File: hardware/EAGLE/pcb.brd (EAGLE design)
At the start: 17.8 x 110.5 mm, 44 parts, among them IC1 4017N, IC2 DG412DJD, IC3 DG412DJD, Q1 MMBT3904, Q2 MMBT3904, Q3 MMBT3904, Q4 MMBT3904

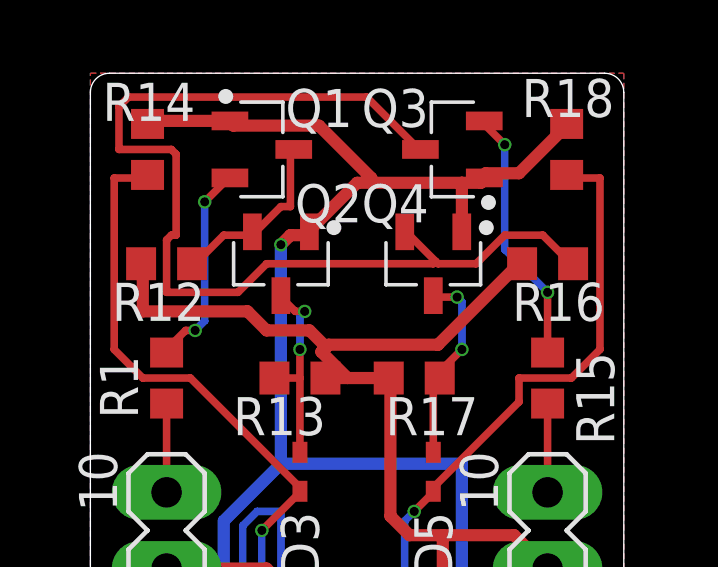
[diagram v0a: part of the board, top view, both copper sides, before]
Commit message: up
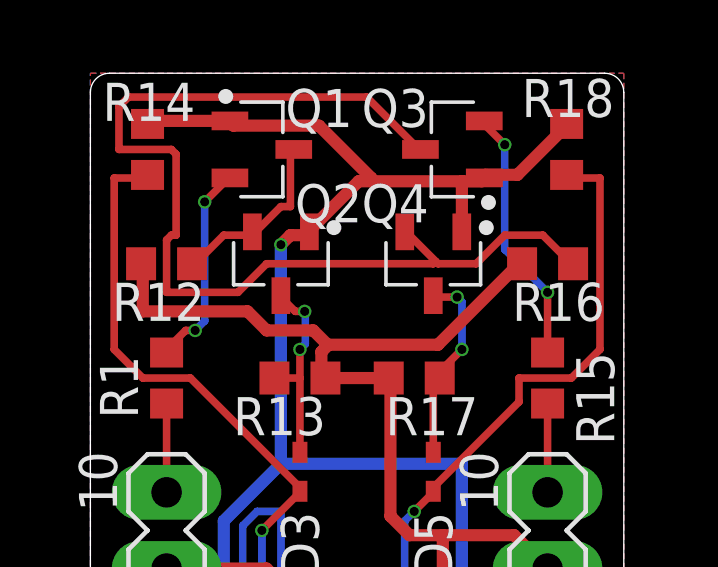
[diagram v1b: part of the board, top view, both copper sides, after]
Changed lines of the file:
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@@
 <contactref element="C4" pad="1"/>
 <contactref element="SV2" pad="9"/>
-<wire x1="11.215" y1="109.22" x2="9.8425" y2="109.22" width="0.4064" layer="1"/>
-<wire x1="9.8425" y1="109.22" x2="9.105" y2="109.22" width="0.4064" layer="1"/>
+<wire x1="11.215" y1="109.22" x2="9.105" y2="109.22" width="0.4064" layer="1"/>
 <wire x1="3.01625" y1="111.4425" x2="3.01625" y2="113.03" width="0.4064" layer="1"/>
 <wire x1="6.50875" y1="111.4425" x2="3.01625" y2="111.4425" width="0.4064" layer="1"/>
 <wire x1="7.14375" y1="110.8075" x2="6.50875" y2="111.4425" width="0.4064" layer="1"/>
-<wire x1="8.5725" y1="110.8075" x2="7.14375" y2="110.8075" width="0.4064" layer="1"/>
-<wire x1="9.8425" y1="109.22" x2="8.969375" y2="110.093125" width="0.4064" layer="1"/>
-<wire x1="9.128125" y1="110.251875" x2="8.5725" y2="110.8075" width="0.4064" layer="1"/>
+<wire x1="8.6995" y1="110.8075" x2="7.14375" y2="110.8075" width="0.4064" layer="1"/>
+<wire x1="9.191625" y1="110.315375" x2="8.6995" y2="110.8075" width="0.4064" layer="1"/>
 <wire x1="3.01625" y1="113.03" x2="2.96" y2="113.03" width="0.4064" layer="1"/>
 <wire x1="12.85875" y1="110.33125" x2="15.5575" y2="113.03" width="0.4064" layer="1"/>
 <wire x1="9.2075" y1="110.33125" x2="12.85875" y2="110.33125" width="0.4064" layer="1"/>
 <wire x1="15.5575" y1="113.03" x2="15.66" y2="113.03" width="0.4064" layer="1"/>
-<wire x1="9.2075" y1="110.33125" x2="9.128125" y2="110.251875" width="0.4064" layer="1"/>
-<wire x1="9.128125" y1="110.251875" x2="8.969375" y2="110.093125" width="0.4064" layer="1"/>
+<wire x1="9.2075" y1="110.33125" x2="9.191625" y2="110.315375" width="0.4064" layer="1"/>
+<wire x1="9.191625" y1="110.315375" x2="8.969375" y2="110.093125" width="0.4064" layer="1"/>
 <wire x1="15.39875" y1="103.98125" x2="16.51" y2="102.87" width="0.4064" layer="1"/>
 <wire x1="11.90625" y1="103.98125" x2="13.0175" y2="103.98125" width="0.4064" layer="1"/>
@@
 <via x="13.0175" y="78.58125" extent="1-16" drill="0.3"/>
 <via x="14.2875" y="77.31125" extent="1-16" drill="0.3"/>
+<wire x1="8.969375" y1="110.093125" x2="8.969375" y2="109.355625" width="0.4064" layer="1"/>
+<wire x1="8.969375" y1="109.355625" x2="9.105" y2="109.22" width="0.4064" layer="1"/>
 </signal>
 <signal name="-12V" class="1">
@@
 <wire x1="8.09625" y1="111.4425" x2="7.62" y2="111.91875" width="0.254" layer="1"/>
 <wire x1="8.41375" y1="111.4425" x2="8.09625" y2="111.4425" width="0.254" layer="1"/>
-<wire x1="8.255" y1="111.28375" x2="8.41375" y2="111.4425" width="0.254" layer="16"/>
-<wire x1="8.255" y1="110.1725" x2="8.255" y2="111.28375" width="0.254" layer="16"/>
+<wire x1="8.41375" y1="111.4425" x2="8.4328" y2="111.42345" width="0.254" layer="16"/>
+<wire x1="8.4328" y1="111.42345" x2="8.4328" y2="110.3503" width="0.254" layer="16"/>
+<wire x1="8.255" y1="110.1725" x2="8.4328" y2="110.3503" width="0.254" layer="16"/>
 <wire x1="8.255" y1="109.22" x2="8.255" y2="110.1725" width="0.254" layer="1"/>
 <wire x1="7.62" y1="111.91875" x2="7.62" y2="111.966" width="0.254" layer="1"/>
@@
 <wire x1="3.175" y1="117.7925" x2="3.175" y2="117.69" width="0.4064" layer="1"/>
 <wire x1="5.87375" y1="117.7925" x2="5.921" y2="117.79" width="0.4064" layer="1"/>
-<wire x1="15.5575" y1="116.04625" x2="17.145" y2="117.63375" width="0.4064" layer="1"/>
-<wire x1="14.44625" y1="116.04625" x2="15.5575" y2="116.04625" width="0.4064" layer="1"/>
+<wire x1="15.5067" y1="115.99545" x2="17.145" y2="117.63375" width="0.4064" layer="1"/>
+<wire x1="14.4308875" y1="115.99545" x2="15.5067" y2="115.99545" width="0.4064" layer="1"/>
 <wire x1="17.145" y1="117.63375" x2="17.145" y2="117.69" width="0.4064" layer="1"/>
-<wire x1="14.44625" y1="116.04625" x2="14.399" y2="115.89" width="0.4064" layer="1"/>
-<wire x1="10.16" y1="115.72875" x2="8.5725" y2="114.14125" width="0.4064" layer="1"/>
-<wire x1="14.2875" y1="115.72875" x2="13.6525" y2="115.72875" width="0.4064" layer="1"/>
-<wire x1="13.6525" y1="115.72875" x2="10.63625" y2="115.72875" width="0.4064" layer="1"/>
-<wire x1="10.63625" y1="115.72875" x2="10.16" y2="115.72875" width="0.4064" layer="1"/>
+<wire x1="14.4308875" y1="115.99545" x2="14.399" y2="115.89" width="0.4064" layer="1"/>
+<wire x1="10.2108" y1="115.77955" x2="8.5725" y2="114.14125" width="0.4064" layer="1"/>
+<wire x1="14.322628125" y1="115.77955" x2="13.6525" y2="115.77955" width="0.4064" layer="1"/>
+<wire x1="13.6525" y1="115.77955" x2="10.63625" y2="115.77955" width="0.4064" layer="1"/>
+<wire x1="10.63625" y1="115.77955" x2="10.2108" y2="115.77955" width="0.4064" layer="1"/>
 <wire x1="8.5725" y1="114.14125" x2="8.57" y2="114.094" width="0.4064" layer="1"/>
-<wire x1="14.2875" y1="115.72875" x2="14.399" y2="115.89" width="0.4064" layer="1"/>
-<wire x1="13.6525" y1="115.72875" x2="13.6525" y2="114.14125" width="0.4064" layer="1"/>
+<wire x1="14.322628125" y1="115.77955" x2="14.399" y2="115.89" width="0.4064" layer="1"/>
+<wire x1="13.6525" y1="115.77955" x2="13.6525" y2="114.14125" width="0.4064" layer="1"/>
 <wire x1="13.6525" y1="114.14125" x2="13.65" y2="114.094" width="0.4064" layer="1"/>
 <wire x1="8.89" y1="117.63375" x2="6.0325" y2="117.63375" width="0.4064" layer="1"/>
 <wire x1="10.63625" y1="115.8875" x2="8.89" y2="117.63375" width="0.4064" layer="1"/>
 <wire x1="6.0325" y1="117.63375" x2="5.921" y2="117.79" width="0.4064" layer="1"/>
-<wire x1="10.63625" y1="115.8875" x2="10.63625" y2="115.72875" width="0.4064" layer="1"/>
+<wire x1="10.63625" y1="115.8875" x2="10.63625" y2="115.77955" width="0.4064" layer="1"/>
 <wire x1="5.715" y1="102.87" x2="3.81" y2="102.87" width="0.4064" layer="16"/>
 <wire x1="5.715" y1="104.4575" x2="5.715" y2="102.87" width="0.4064" layer="16"/>
